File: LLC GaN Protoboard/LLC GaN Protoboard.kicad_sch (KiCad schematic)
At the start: 0 parts

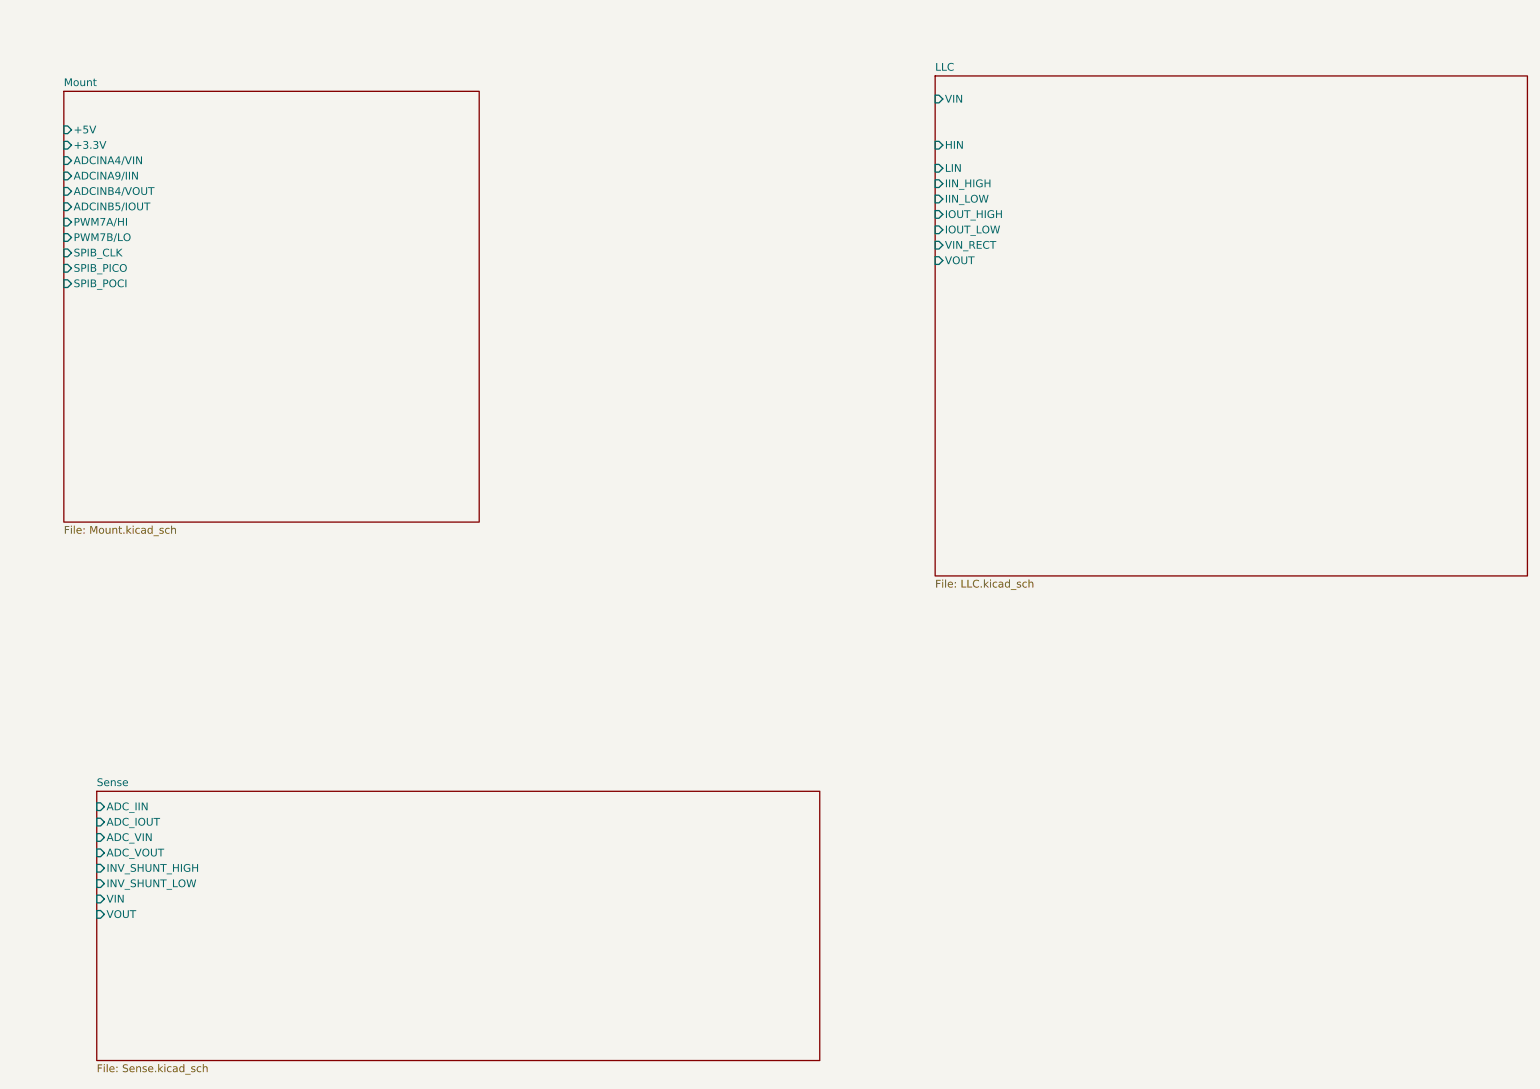
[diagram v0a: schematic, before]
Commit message: Edited schematic
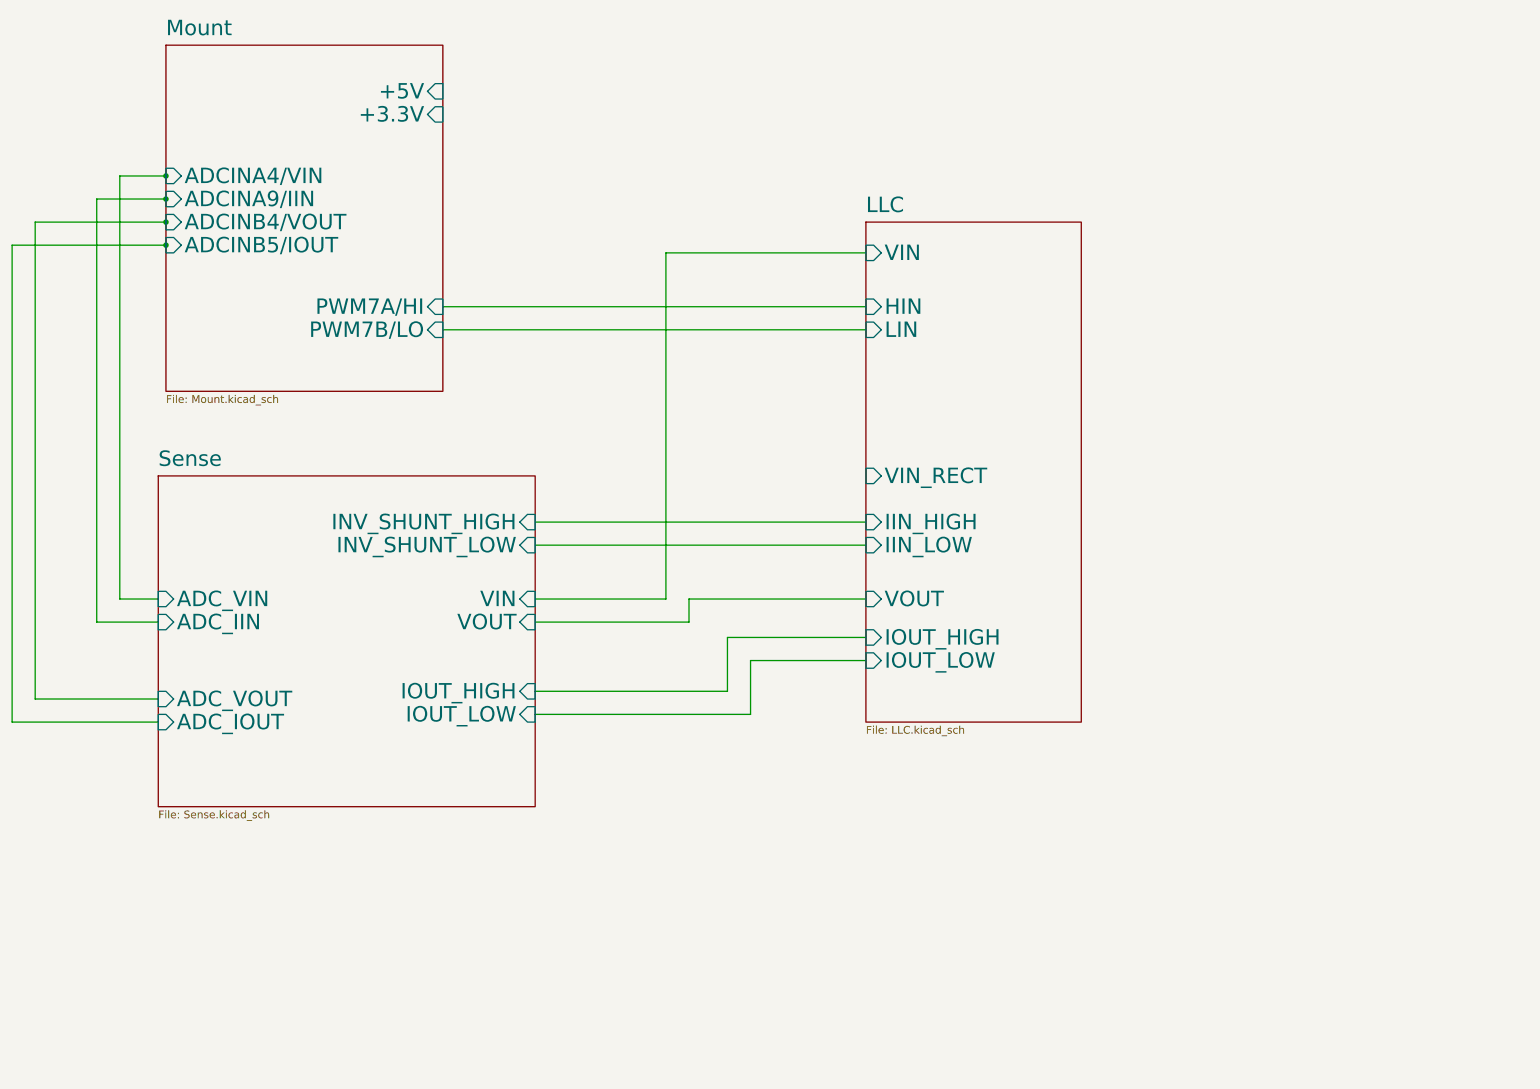
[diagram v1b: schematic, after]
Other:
- sheet Mount ports: added none; removed SPIB_CLK, SPIB_PICO, SPIB_POCI
- sheet Sense ports: added IOUT_HIGH, IOUT_LOW; removed none

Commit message: first route
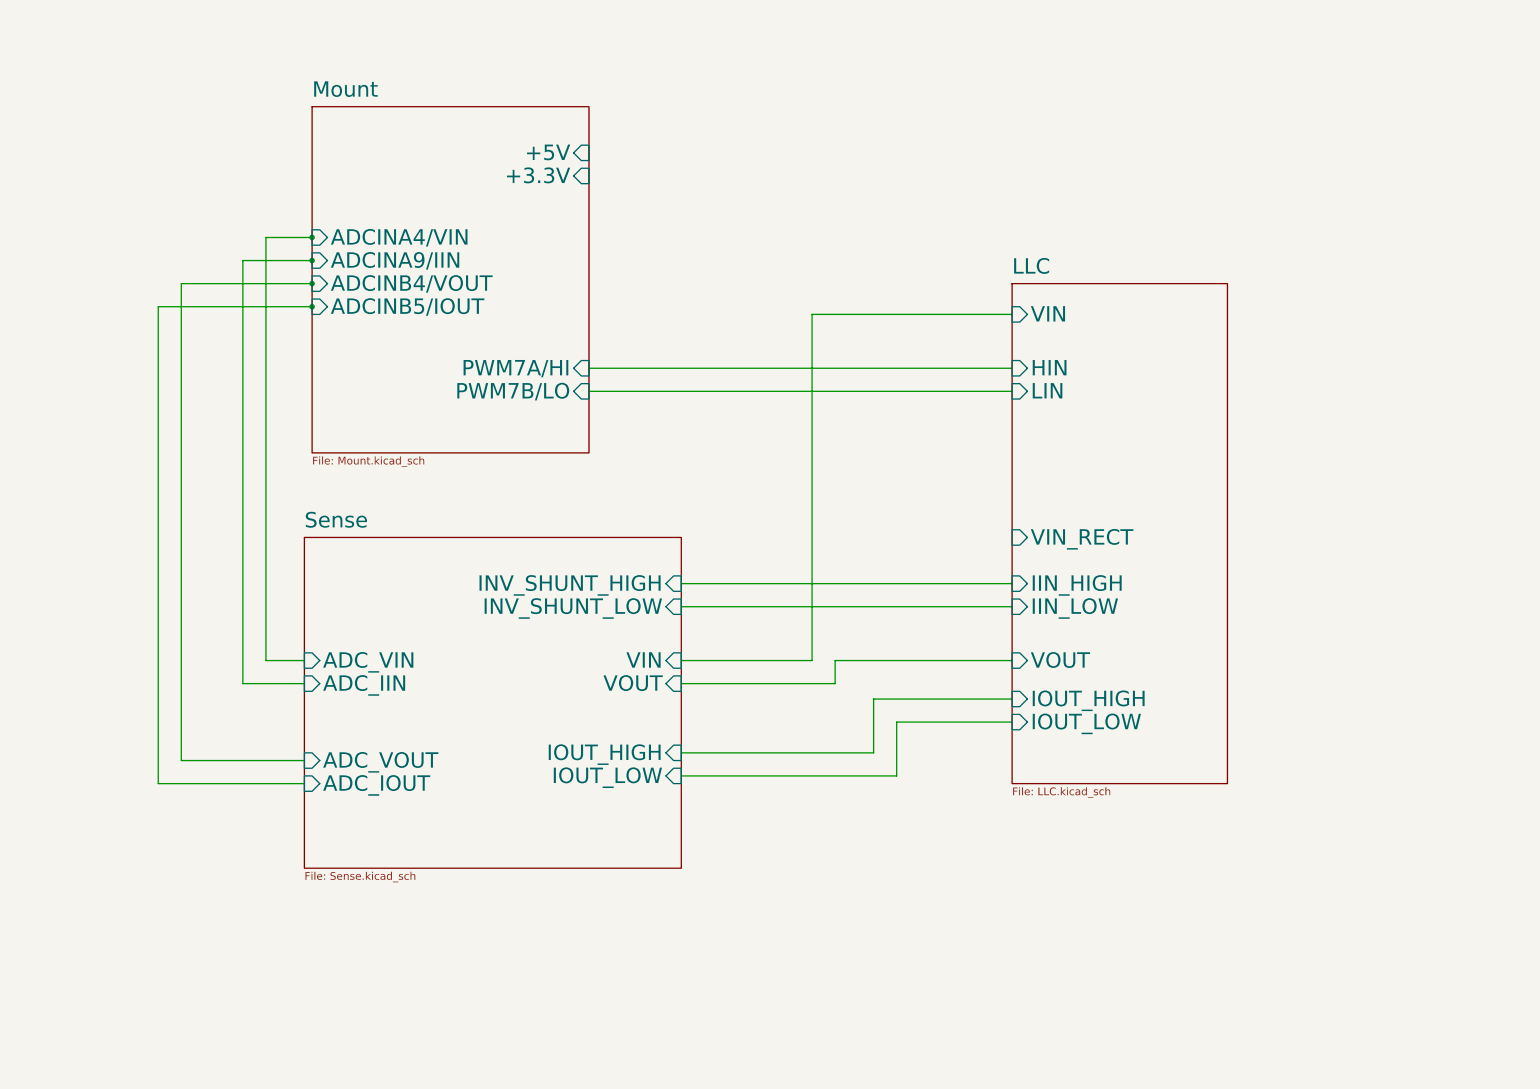
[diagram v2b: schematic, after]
